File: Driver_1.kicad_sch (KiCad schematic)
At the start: 34 parts

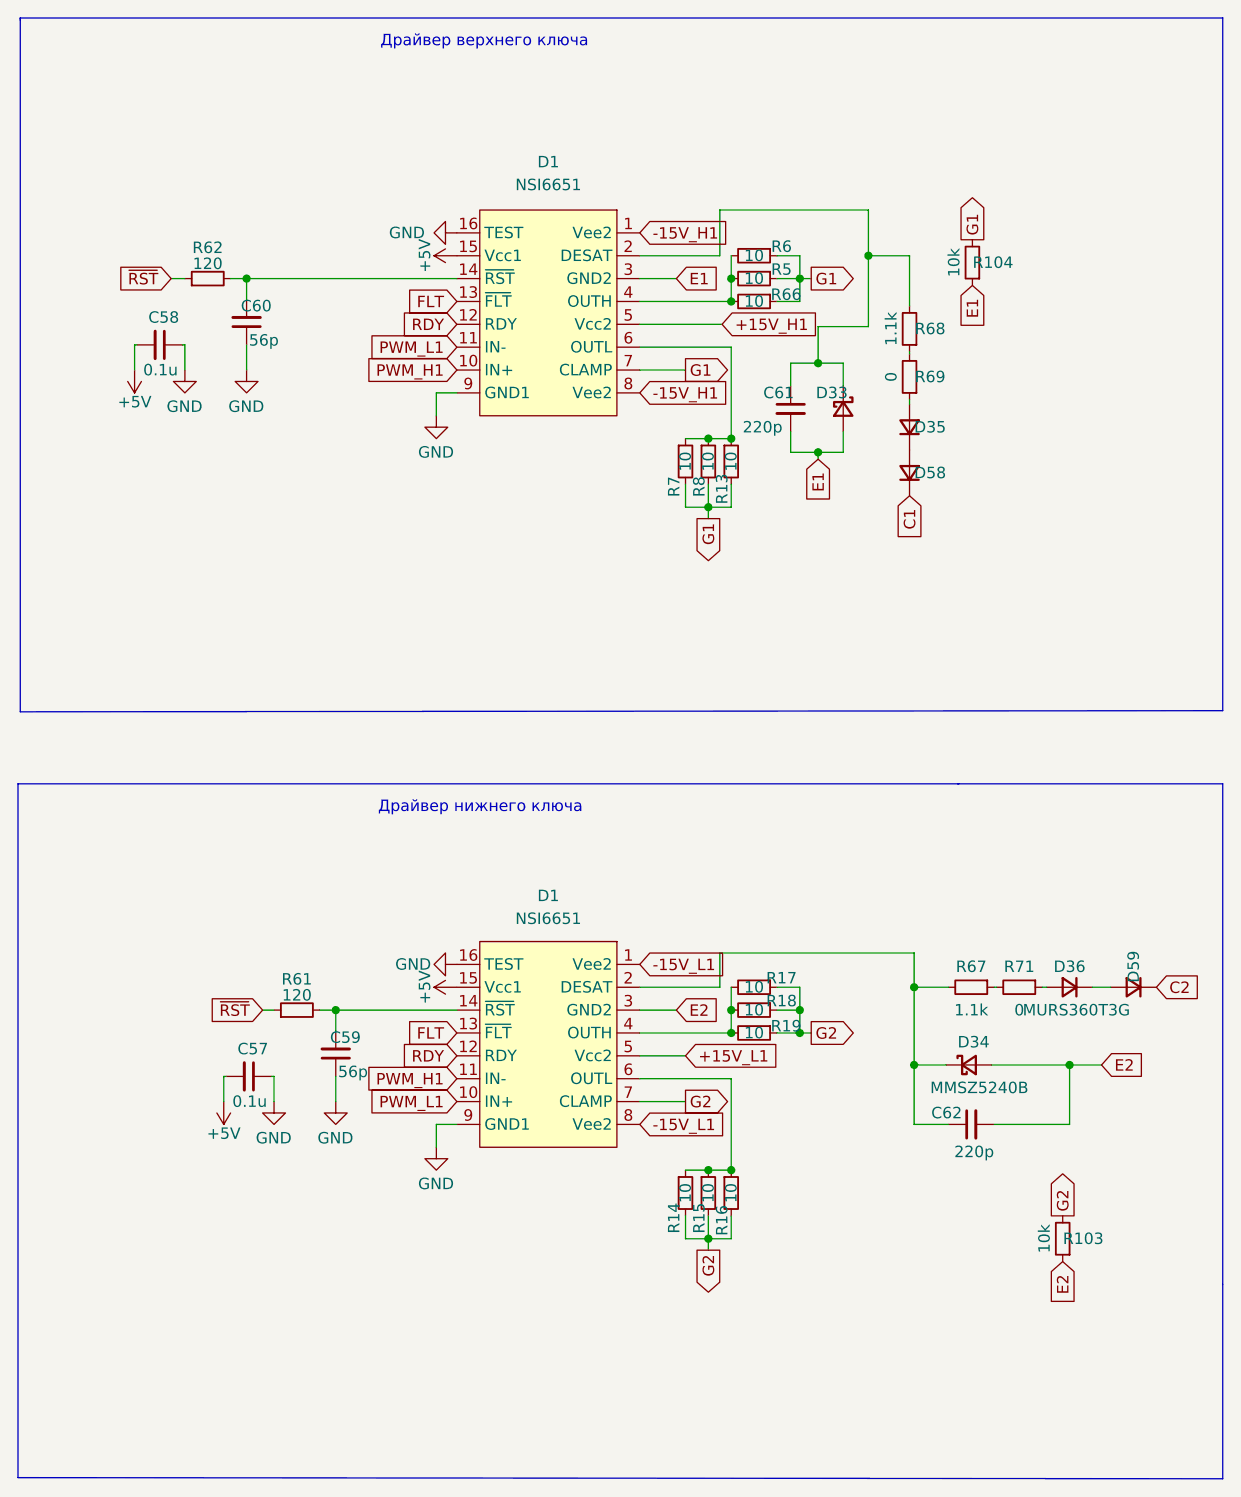
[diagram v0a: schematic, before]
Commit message: Развел вторую стойку
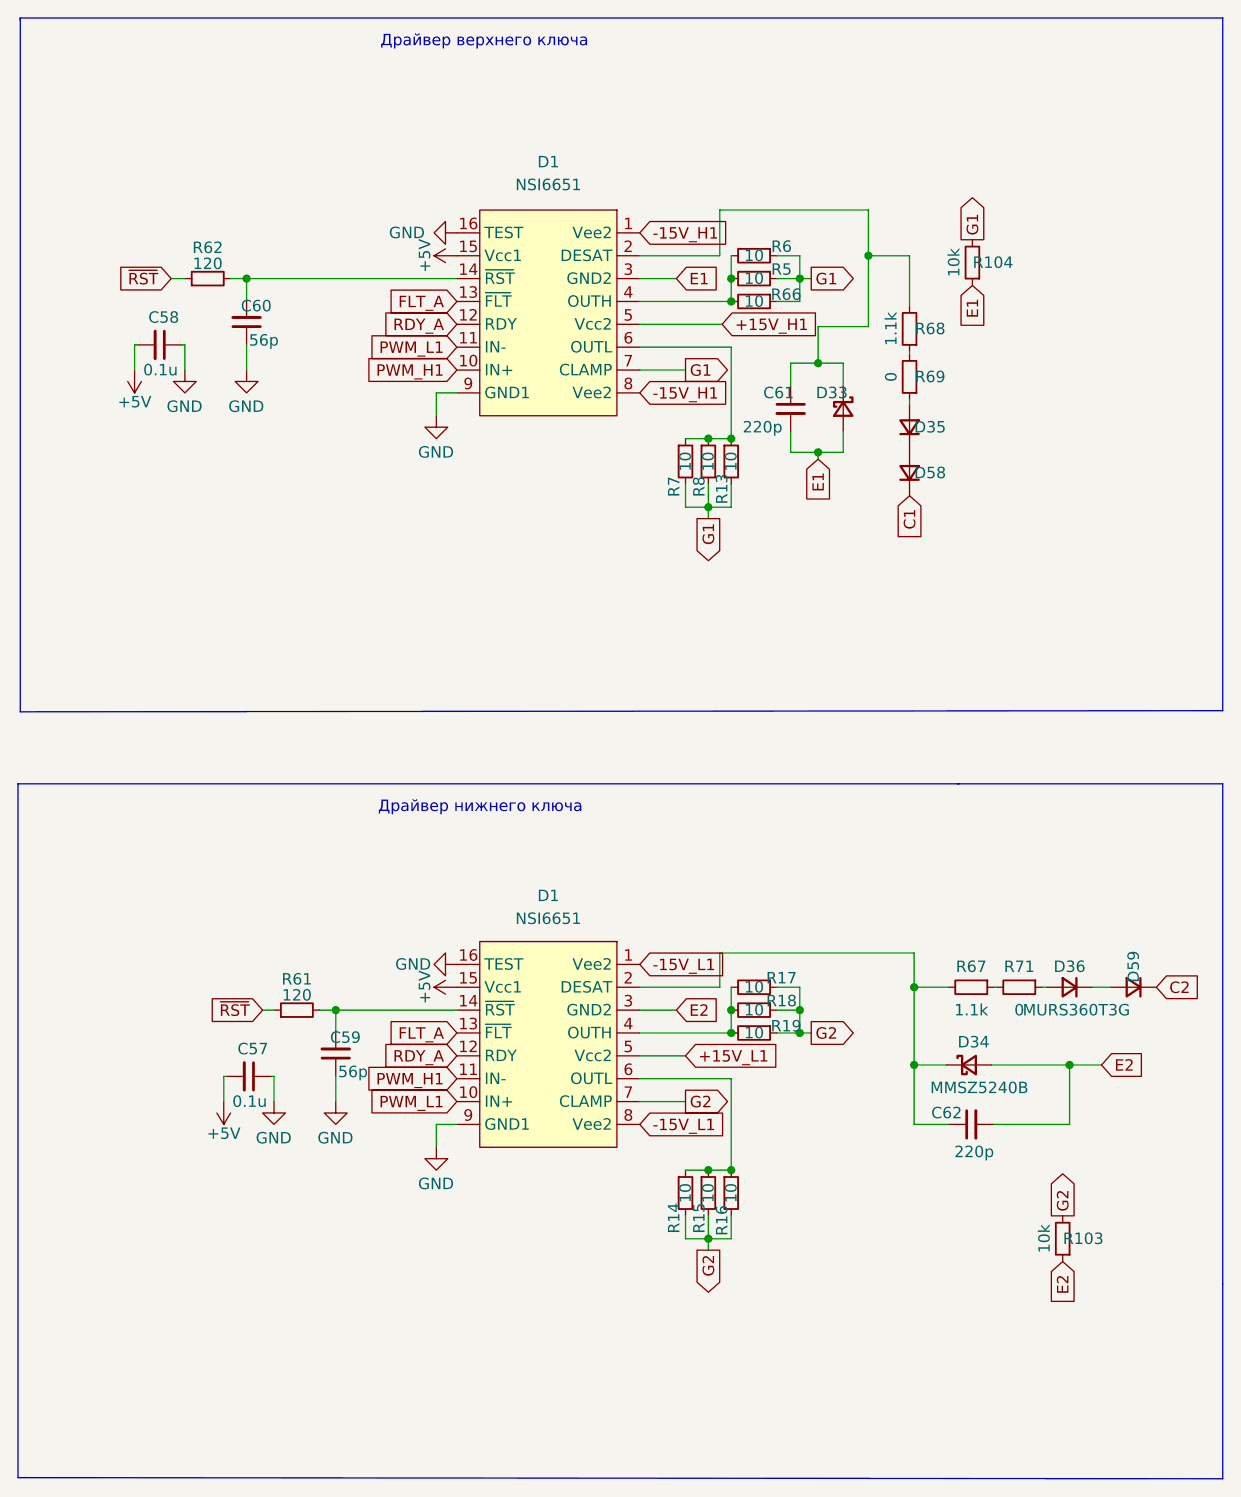
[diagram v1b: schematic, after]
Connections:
- net FLT renamed FLT_A
- net RDY renamed RDY_A
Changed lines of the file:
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@@
 		)
 	)
-	(global_label "RDY"
+	(global_label "RDY_A"
 		(shape input)
 		(at 80.01 57.15 180)
@@
 		)
 		(property "Intersheetrefs" "${INTERSHEET_REFS}"
-			(at 74.0684 57.15 0)
+			(at 71.34 57.15 0)
 			(effects
 				(font
@@
 		)
 	)
-	(global_label "FLT"
+	(global_label "FLT_A"
 		(shape input)
 		(at 80.01 54.61 180)
@@
 		)
 		(property "Intersheetrefs" "${INTERSHEET_REFS}"
-			(at 74.4506 54.61 0)
-			(effects
-				(font
-					(size 1.27 1.27)
-				)
-				(justify right)
-				(hide yes)
-			)
-		)
-	)
-	(global_label "FLT"
+			(at 71.8843 54.61 0)
+			(effects
+				(font
+					(size 1.27 1.27)
+				)
+				(justify right)
+				(hide yes)
+			)
+		)
+	)
+	(global_label "FLT_A"
 		(shape input)
 		(at 80.01 135.89 180)
@@
 		)
 		(property "Intersheetrefs" "${INTERSHEET_REFS}"
-			(at 74.4506 135.89 0)
+			(at 71.8843 135.89 0)
 			(effects
 				(font
@@
 		)
 	)
-	(global_label "RDY"
+	(global_label "RDY_A"
 		(shape input)
 		(at 80.01 138.43 180)
@@
 		)
 		(property "Intersheetrefs" "${INTERSHEET_REFS}"
-			(at 74.0684 138.43 0)
-			(effects
-				(font
+			(at 71.34 138.43 0)
+			(effects
+				(font
